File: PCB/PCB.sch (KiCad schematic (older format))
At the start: 44 parts, among them J1 USB_B, J10 Vapor maker, J11 chamber LED, J2 power 12V, J3 DS18B20, J4 NEXTION 2.8\", J5 4pin FAN, J6 4pin FAN, J7 4pin FAN, J8 Peltiers 12V, J9 Peltiers 3.3V, Q1 IRF530N, Q10 IRFD110, Q11 IRFD110, Q12 IRFD110, Q13 IRFD110, Q14 IRFD110, Q15 IRF530N, Q2 IRF530N, Q3 IRF530N, Q4 IRF530N, Q5 IRF530N, Q6 IRF530N, Q7 IRFD110, Q8 IRFD110, Q9 IRFD110, U1 CH340G, U2 ESP32-WROOM-32, U3 LF33CDT, U4 L7805, Y1 12MHz

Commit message: PCB General UPGRADE
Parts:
- removed J11: chamber LED, TerminalBlock_WAGO:TerminalBlock_WAGO_804-102_1x02_P5.00mm_45Degree, symbol Connector_Generic:Conn_01x02
- removed Q10, Q11, Q12, Q13, Q14, Q7, Q8, Q9: IRFD110, Package_DIP:Vishay_HVM-DIP-3_W7.62mm, symbol Transistor_FET:IRF40DM229
- removed Q15: IRF530N, Package_TO_SOT_THT:TO-220-3_Vertical, symbol Transistor_FET:IRF540N
- added H1, H2, H3, H4: MountingHole_Pad, MountingHole:MountingHole_3.2mm_M3_Pad_Via, symbol Mechanical:MountingHole_Pad
- added J11: LED + Pump, TerminalBlock_WAGO:TerminalBlock_WAGO_236-104_1x04_P5.00mm_45Degree, symbol Connector_Generic:Conn_01x04
- added J12: I2C, Connector_PinHeader_2.54mm:PinHeader_1x04_P2.54mm_Horizontal, symbol Connector_Generic:Conn_01x04
- added Q10, Q11, Q12, Q13, Q14, Q15, Q7, Q8, Q9: TSM2302, Package_TO_SOT_SMD:SOT-23, symbol Transistor_FET:ZXMN2A01F
- added Q16, Q17: IRF530N, Package_TO_SOT_THT:TO-220-3_Vertical, symbol Transistor_FET:IRF540N
- added R8: 5k6, Resistor_SMD:R_1206_3216Metric_Pad1.42x1.75mm_HandSolder, symbol Device:R
- J10, J8, J9: footprint Connector_Phoenix_GMSTB:PhoenixContact_GMSTBVA_2,5_4-G-7,62_1x04_P7.62mm_Vertical -> TerminalBlock_WAGO:TerminalBlock_WAGO_236-104_1x04_P5.00mm_45Degree
- R1, R2, R3, R4, R5, R6, R7: footprint Resistor_THT:R_Axial_DIN0207_L6.3mm_D2.5mm_P10.16mm_Horizontal -> Resistor_SMD:R_1206_3216Metric_Pad1.42x1.75mm_HandSolder
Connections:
- wire segments 193 -> 212

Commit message: pcb update
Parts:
- removed C3, C6: 0.1uF, Capacitor_SMD:C_1206_3216Metric, symbol Device:C
- removed C4: 2.2uF, Capacitor_THT:CP_Radial_D5.0mm_P2.00mm, symbol Device:CP
- removed C5: 0.33uF, Capacitor_SMD:C_1206_3216Metric, symbol Device:C
- removed H1, H2, H3, H4: MountingHole_Pad, MountingHole:MountingHole_3.2mm_M3_Pad_Via, symbol Mechanical:MountingHole_Pad
- removed J10: Vapor maker, TerminalBlock_WAGO:TerminalBlock_WAGO_236-104_1x04_P5.00mm_45Degree, symbol Connector_Generic:Conn_01x04
- removed J11: LED + Pump, TerminalBlock_WAGO:TerminalBlock_WAGO_236-104_1x04_P5.00mm_45Degree, symbol Connector_Generic:Conn_01x04
- removed J12: I2C, Connector_PinHeader_2.54mm:PinHeader_1x04_P2.54mm_Horizontal, symbol Connector_Generic:Conn_01x04
- removed J2: power 12V, Connector_PinHeader_2.54mm:PinHeader_1x03_P2.54mm_Horizontal, symbol Connector_Generic:Conn_01x03
- removed J3: DS18B20, Connector_PinHeader_2.54mm:PinHeader_1x03_P2.54mm_Horizontal, symbol Connector_Generic:Conn_01x03
- removed J4: NEXTION 2.8\", Connector_PinHeader_2.54mm:PinHeader_1x04_P2.54mm_Horizontal, symbol Connector_Generic:Conn_01x04
- removed J5, J6, J7: 4pin FAN, Connector:FanPinHeader_1x04_P2.54mm_Vertical, symbol Connector_Generic:Conn_01x04
- removed J8: Peltiers 12V, TerminalBlock_WAGO:TerminalBlock_WAGO_236-104_1x04_P5.00mm_45Degree, symbol Connector_Generic:Conn_01x04
- removed J9: Peltiers 3.3V, TerminalBlock_WAGO:TerminalBlock_WAGO_236-104_1x04_P5.00mm_45Degree, symbol Connector_Generic:Conn_01x04
- removed Q1, Q16, Q17, Q2, Q3, Q4, Q5, Q6: IRF530N, Package_TO_SOT_THT:TO-220-3_Vertical, symbol Transistor_FET:IRF540N
- removed Q10, Q11, Q12, Q13, Q14, Q15, Q7, Q8, Q9: TSM2302, Package_TO_SOT_SMD:SOT-23, symbol Transistor_FET:ZXMN2A01F
- removed R1, R2, R3, R4, R5, R6, R7, R8: 5k6, Resistor_SMD:R_1206_3216Metric_Pad1.42x1.75mm_HandSolder, symbol Device:R
- removed U1: CH340G, Package_SO:SOP-16_4.4x10.4mm_P1.27mm, symbol Interface_USB:CH340G
- removed U2: ESP32-WROOM-32, RF_Module:ESP32-WROOM-32, symbol RF_Module:ESP32-WROOM-32
- removed U3: LF33CDT, Package_TO_SOT_SMD:TO-252-2, symbol Regulator_Linear:LF33_TO220
- removed U4: L7805, Package_TO_SOT_SMD:TO-252-2, symbol Regulator_Linear:L7805
- removed Y1: 12MHz, Crystal:Crystal_HC49-U_Vertical, symbol Device:Crystal
- added CH340G1: CH340G, Package_SO:SOIC-16_3.9x9.9mm_P1.27mm, symbol Interface_USB:CH340G
- added U1: ESP32-WROOM-32, RF_Module:ESP32-WROOM-32, symbol RF_Module:ESP32-WROOM-32
- added X1: 12MHz, Crystals:Crystal_SMD_HC49-SD_HandSoldering, symbol Device:Crystal
- added power_12V1: Conn_01x03, Mlab_Pin_Headers:Straight_2x03, symbol Connector_Generic:Conn_01x03
- C1, C2: value 22pF -> 22p; footprint Capacitor_SMD:C_1206_3216Metric -> Capacitors_SMD:C_1206_HandSoldering
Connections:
- net labels added: +12V, +3.3V, +5V, DTR, RTS, RXD, TXD, usb_N, usb_P
- wire segments 212 -> 37

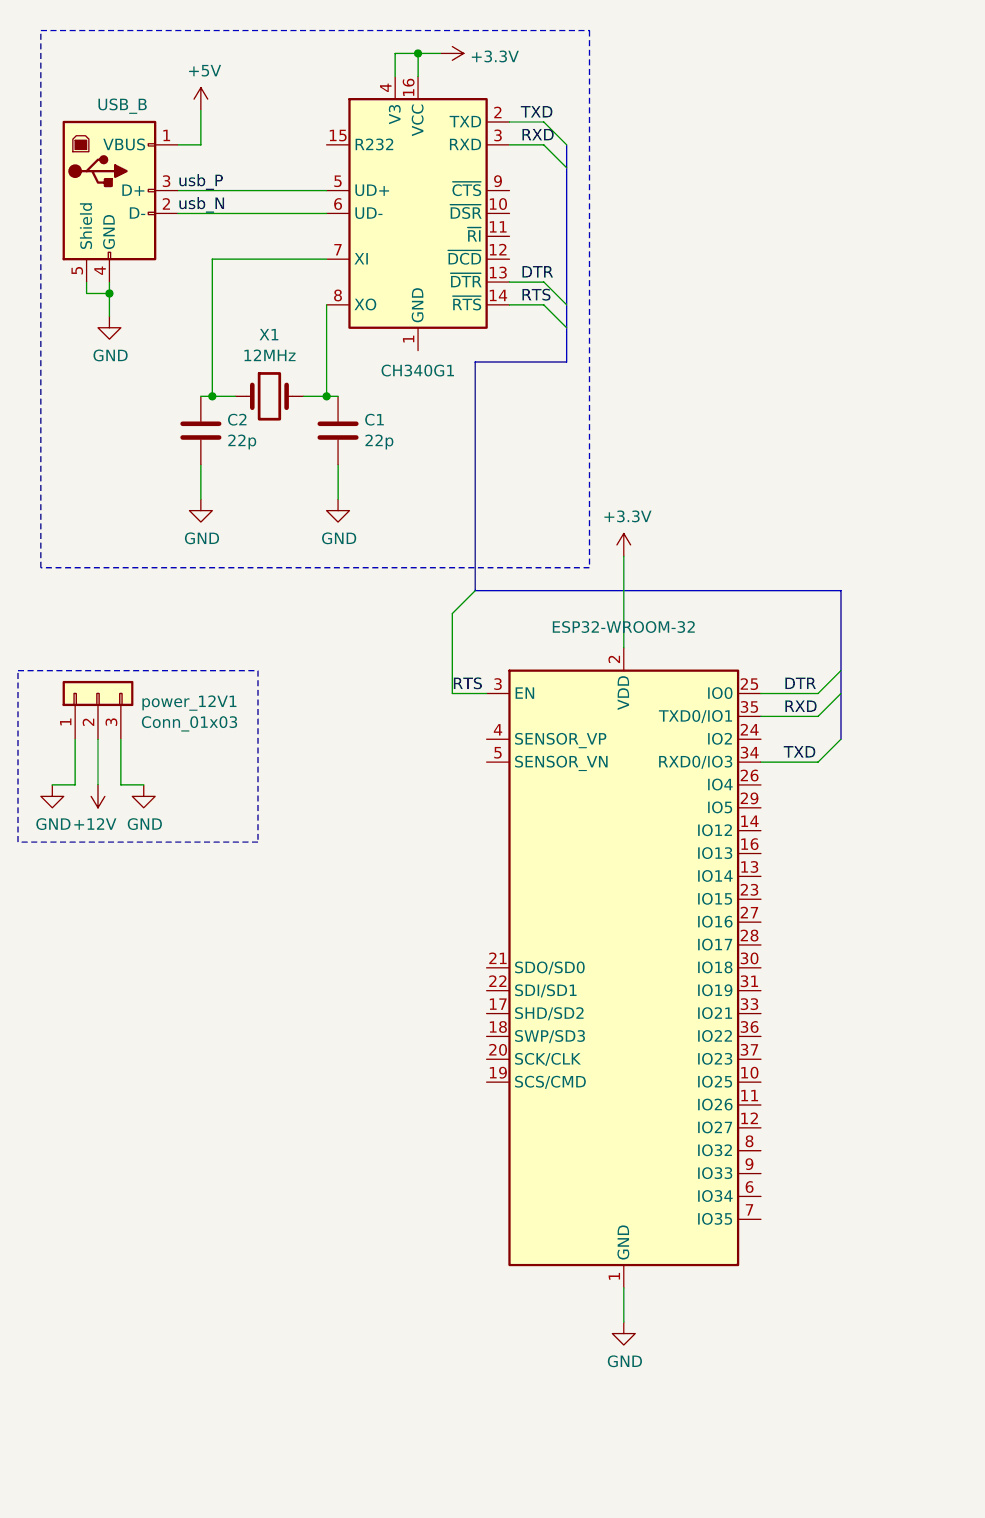
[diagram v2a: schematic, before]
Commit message: pcb
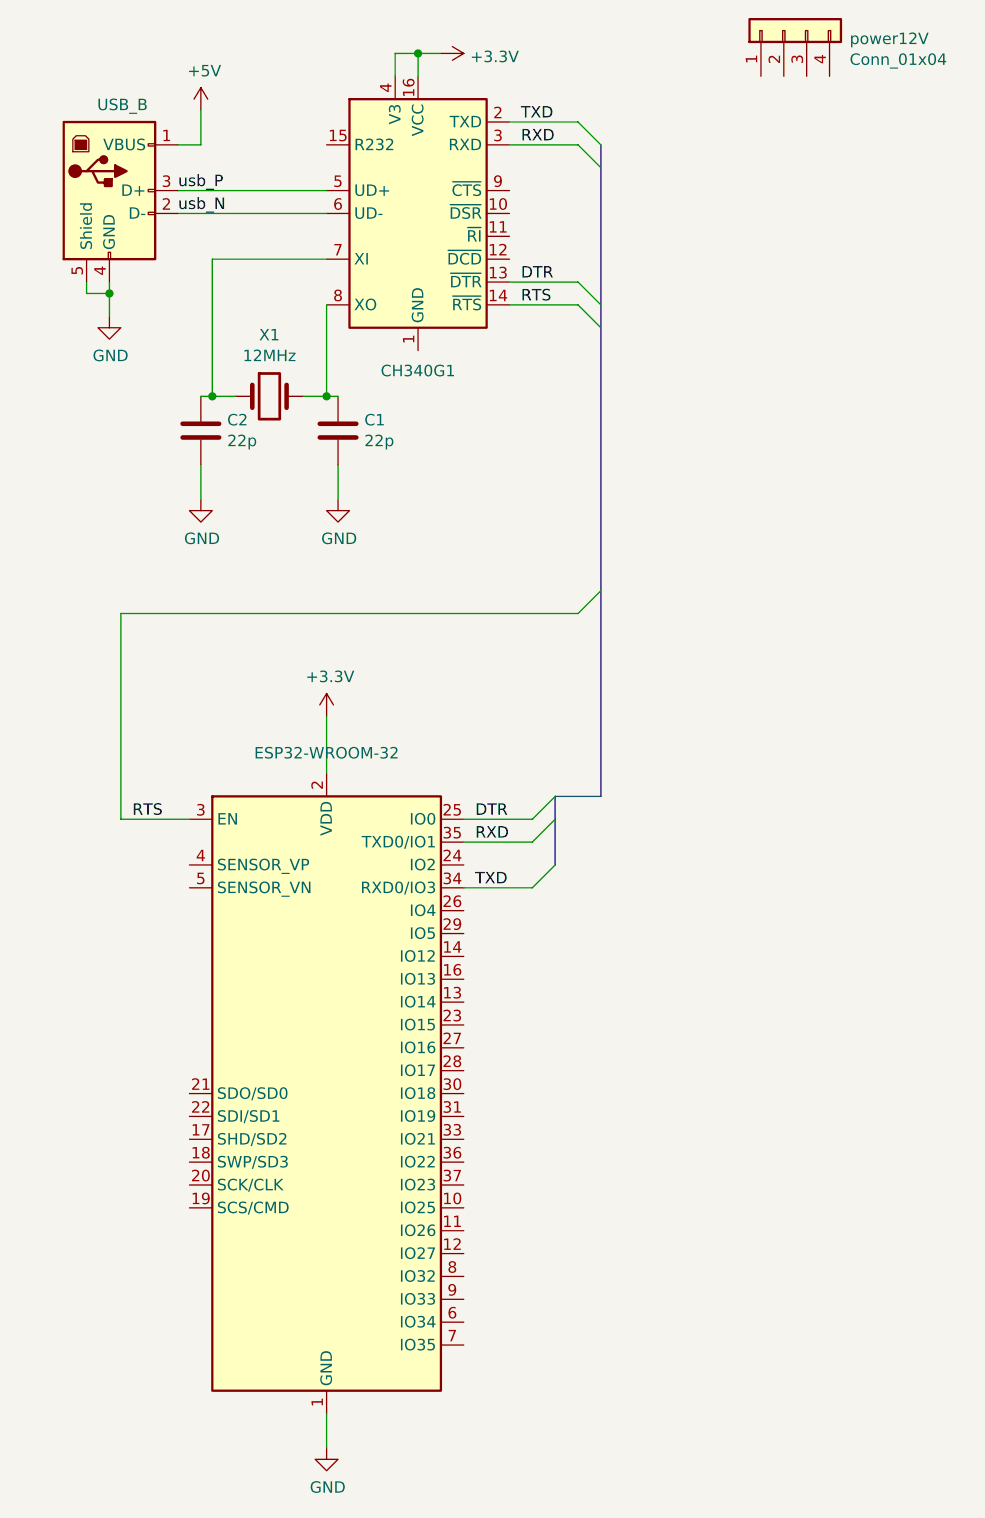
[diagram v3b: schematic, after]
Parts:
- removed power_12V1: Conn_01x03, Mlab_Pin_Headers:Straight_2x03, symbol Connector_Generic:Conn_01x03
- added power12V: Conn_01x04, Mlab_Pin_Headers:Straight_2x04, symbol Connector_Generic:Conn_01x04
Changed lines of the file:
@@
 EESchema Schematic File Version 4
-LIBS:PCB-cache
 EELAYER 30 0
 EELAYER END
@@
 usb_N
 $Comp
-L RF_Module:ESP32-WROOM-32 U1
-U 1 1 5DA32DFA
-P 3700 5150
-F 0 "U1" H 3700 6731 50  0001 C CNN
-F 1 "ESP32-WROOM-32" H 3700 6639 50  0000 C CNN
-F 2 "RF_Module:ESP32-WROOM-32" H 3700 3650 50  0001 C CNN
-F 3 "https://www.espressif.com/sites/default/files/documentation/esp32-wroom-32_datasheet_en.pdf" H 3400 5200 50  0001 C CNN
-	1    3700 5150
-	1    0    0    -1
-$EndComp
-$Comp
 L Device:Crystal X1
 U 1 1 5DA400F9
@@
 Wire Wire Line
 	1450 2200 1450 2150
-Entry Wire Line
-	3350 1450 3450 1550
-Entry Wire Line
-	3350 1550 3450 1650
-Entry Wire Line
-	3350 2150 3450 2250
-Entry Wire Line
-	3350 2250 3450 2350
-Wire Wire Line
-	3200 1450 3350 1450
-Wire Wire Line
-	3200 1550 3350 1550
-Wire Wire Line
-	3200 2150 3350 2150
-Wire Wire Line
-	3200 2250 3350 2250
-Text Label 3250 1450 0    50   ~ 0
-TXD
-Text Label 3250 1550 0    50   ~ 0
-RXD
-Text Label 3250 2150 0    50   ~ 0
-DTR
-Text Label 3250 2250 0    50   ~ 0
-RTS
-Wire Wire Line
-	3100 3950 2950 3950
-Wire Wire Line
-	2950 3950 2950 3600
-Entry Wire Line
-	2950 3600 3050 3500
-Wire Wire Line
-	4300 4050 4550 4050
-Wire Wire Line
-	4300 4250 4550 4250
-Entry Wire Line
-	4550 4050 4650 3950
-Entry Wire Line
-	4550 4250 4650 4150
-Wire Bus Line
-	4650 3500 3050 3500
-Wire Bus Line
-	3050 3500 3050 2500
-Wire Bus Line
-	3050 2500 3450 2500
-Text Label 4400 4250 0    50   ~ 0
-TXD
-Text Label 4400 4050 0    50   ~ 0
-RXD
-Text Label 2950 3950 0    50   ~ 0
-RTS
-Wire Wire Line
-	4300 3950 4550 3950
-Entry Wire Line
-	4550 3950 4650 3850
-Text Label 4400 3950 0    50   ~ 0
-DTR
-$Comp
-L power:+3.3V #PWR0108
-U 1 1 5DA62BDB
-P 3700 3350
-F 0 "#PWR0108" H 3700 3200 50  0001 C CNN
-F 1 "+3.3V" H 3715 3523 50  0000 C CNN
-F 2 "" H 3700 3350 50  0001 C CNN
-F 3 "" H 3700 3350 50  0001 C CNN
-	1    3700 3350
-	1    0    0    -1
-$EndComp
-Wire Wire Line
-	3700 3750 3700 3350
-$Comp
-L power:GND #PWR0109
-U 1 1 5DA64609
-P 3700 6700
-F 0 "#PWR0109" H 3700 6450 50  0001 C CNN
-F 1 "GND" H 3705 6527 50  0000 C CNN
-F 2 "" H 3700 6700 50  0001 C CNN
-F 3 "" H 3700 6700 50  0001 C CNN
-	1    3700 6700
-	1    0    0    -1
-$EndComp
-Wire Wire Line
-	3700 6700 3700 6550
-$Comp
-L Connector_Generic:Conn_01x03 power_12V1
-U 1 1 5DA737E0
-P 1400 3950
-F 0 "power_12V1" V 1364 3762 50  0000 R CNN
-F 1 "Conn_01x03" V 1273 3762 50  0000 R CNN
-F 2 "Mlab_Pin_Headers:Straight_2x03" H 1400 3950 50  0001 C CNN
-F 3 "~" H 1400 3950 50  0001 C CNN
-	1    1400 3950
-	0    -1   -1   0
-$EndComp
-$Comp
-L power:+12V #PWR0101
-U 1 1 5DA7649D
-P 1400 4350
-F 0 "#PWR0101" H 1400 4200 50  0001 C CNN
-F 1 "+12V" H 1415 4523 50  0000 C CNN
-F 2 "" H 1400 4350 50  0001 C CNN
-F 3 "" H 1400 4350 50  0001 C CNN
-	1    1400 4350
-	-1   0    0    1
-$EndComp
-$Comp
-L power:GND #PWR0102
-U 1 1 5DA7684F
-P 1600 4350
-F 0 "#PWR0102" H 1600 4100 50  0001 C CNN
-F 1 "GND" H 1605 4177 50  0000 C CNN
-F 2 "" H 1600 4350 50  0001 C CNN
-F 3 "" H 1600 4350 50  0001 C CNN
-	1    1600 4350
-	1    0    0    -1
-$EndComp
-$Comp
-L power:GND #PWR0103
-U 1 1 5DA76A88
-P 1200 4350
-F 0 "#PWR0103" H 1200 4100 50  0001 C CNN
-F 1 "GND" H 1205 4177 50  0000 C CNN
-F 2 "" H 1200 4350 50  0001 C CNN
-F 3 "" H 1200 4350 50  0001 C CNN
-	1    1200 4350
-	1    0    0    -1
-$EndComp
-Wire Wire Line
-	1400 4350 1400 4150
-Wire Wire Line
-	1300 4150 1300 4350
-Wire Wire Line
-	1300 4350 1200 4350
-Wire Wire Line
-	1500 4150 1500 4350
-Wire Wire Line
-	1500 4350 1600 4350
-Wire Notes Line
-	1050 4600 1050 3850
-Wire Notes Line
-	1050 3850 2100 3850
-Wire Notes Line
-	2100 3850 2100 4600
-Wire Notes Line
-	2100 4600 1050 4600
-Wire Notes Line
-	1150 1050 3550 1050
-Wire Notes Line
-	3550 1050 3550 3400
-Wire Notes Line
-	3550 3400 1150 3400
-Wire Notes Line
-	1150 3400 1150 1050
 $Comp
 L power:+3.3V #PWR?
@@
 Wire Wire Line
 	2800 1250 2800 1150
+Connection ~ 2800 1150
+Wire Wire Line
+	2800 1150 2700 1150
+$Comp
+L Connector_Generic:Conn_01x04 power12V
+U 1 1 5DEF05BC
+P 4400 1050
+F 0 "power12V" V 4364 762 50  0000 R CNN
+F 1 "Conn_01x04" V 4273 762 50  0000 R CNN
+F 2 "Mlab_Pin_Headers:Straight_2x04" H 4400 1050 50  0001 C CNN
+F 3 "~" H 4400 1050 50  0001 C CNN
+	1    4400 1050
+	0    -1   -1   0
+$EndComp
+$Comp
+L RF_Module:ESP32-WROOM-32 U1
+U 1 1 5DA32DFA
+P 2400 5700
+F 0 "U1" H 2400 7281 50  0001 C CNN
+F 1 "ESP32-WROOM-32" H 2400 7189 50  0000 C CNN
+F 2 "RF_Module:ESP32-WROOM-32" H 2400 4200 50  0001 C CNN
+F 3 "https://www.espressif.com/sites/default/files/documentation/esp32-wroom-32_datasheet_en.pdf" H 2100 5750 50  0001 C CNN
+	1    2400 5700
+	1    0    0    -1
+$EndComp
+$Comp
+L power:GND #PWR0109
+U 1 1 5DA64609
+P 2400 7250
+F 0 "#PWR0109" H 2400 7000 50  0001 C CNN
+F 1 "GND" H 2405 7077 50  0000 C CNN
+F 2 "" H 2400 7250 50  0001 C CNN
+F 3 "" H 2400 7250 50  0001 C CNN
+	1    2400 7250
+	1    0    0    -1
+$EndComp
+Wire Wire Line
+	2400 7250 2400 7100
+Wire Wire Line
+	3000 4500 3300 4500
+Wire Wire Line
+	3000 4600 3300 4600
+Wire Wire Line
+	3000 4800 3300 4800
+Wire Wire Line
+	1800 4500 1500 4500
+Wire Wire Line
+	3200 1450 3500 1450
+Wire Wire Line
+	3200 1550 3500 1550
+Wire Wire Line
+	3200 2150 3500 2150
+Wire Wire Line
+	3200 2250 3500 2250
+Text Label 3250 1450 0    50   ~ 0
+TXD
+Text Label 3250 1550 0    50   ~ 0
+RXD
+Text Label 3250 2150 0    50   ~ 0
+DTR
+Text Label 3250 2250 0    50   ~ 0
+RTS
+Text Label 1550 4500 0    50   ~ 0
+RTS
+Text Label 3050 4500 0    50   ~ 0
+DTR
+Text Label 3050 4600 0    50   ~ 0
+RXD
+Text Label 3050 4800 0    50   ~ 0
+TXD
+Entry Wire Line
+	3300 4800 3400 4700
+Entry Wire Line
+	3300 4600 3400 4500
+Entry Wire Line
+	3300 4500 3400 4400
+Entry Wire Line
+	3500 2250 3600 2350
+Entry Wire Line
+	3500 2150 3600 2250
+Entry Wire Line
+	3500 1550 3600 1650
+Entry Wire Line
+	3500 1450 3600 1550
 Wire Bus Line
-	4650 3500 4650 4150
+	3600 4400 3400 4400
+Wire Wire Line
+	1500 4500 1500 3600
+Entry Wire Line
+	3500 3600 3600 3500
+Wire Wire Line
+	1500 3600 3500 3600
+$Comp
+L power:+3.3V #PWR?
+U 1 1 5DF14F2C
+P 2400 4050
+F 0 "#PWR?" H 2400 3900 50  0001 C CNN
+F 1 "+3.3V" H 2415 4223 50  0000 C CNN
+F 2 "" H 2400 4050 50  0001 C CNN
+F 3 "" H 2400 4050 50  0001 C CNN
+	1    2400 4050
+	1    0    0    -1
+$EndComp
+Wire Wire Line
+	2400 4300 2400 4050
 Wire Bus Line
-	3450 1550 3450 2500
-Connection ~ 2800 1150
-Wire Wire Line
-	2800 1150 2700 1150
+	3400 4400 3400 4700
+Wire Bus Line
+	3600 1550 3600 4400
 $EndSCHEMATC

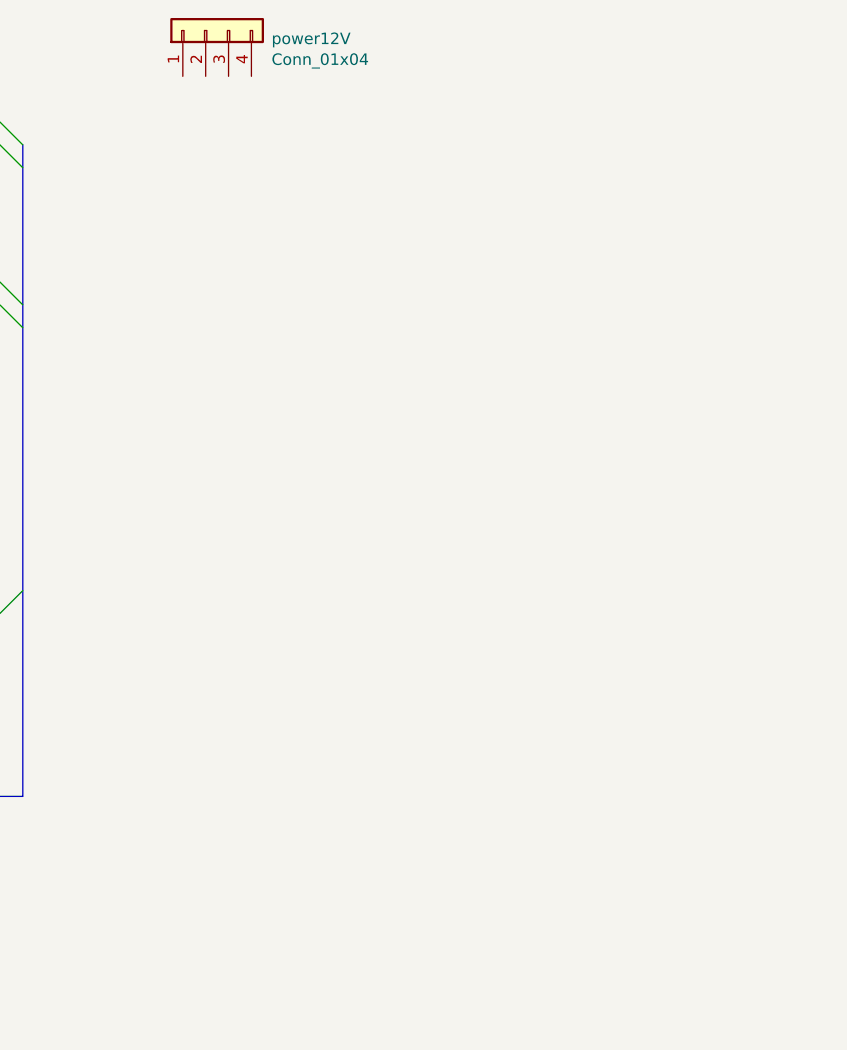
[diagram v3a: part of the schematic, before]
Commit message: pcb, power and 3v3
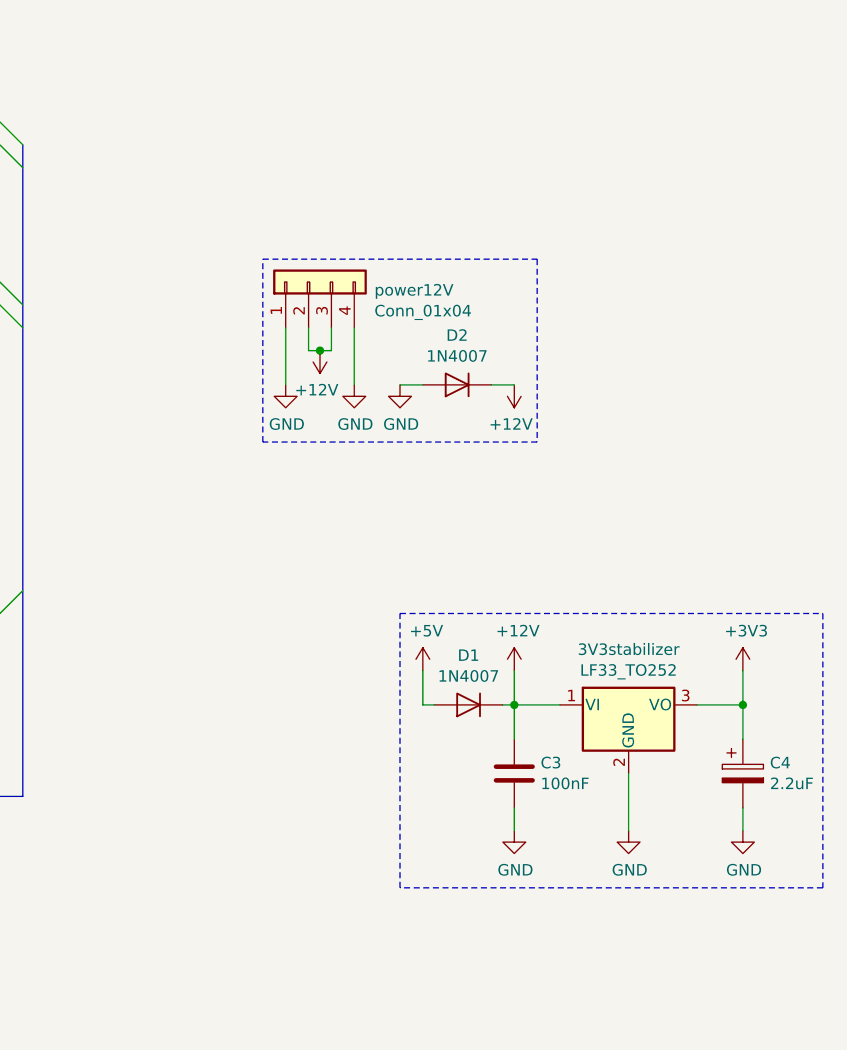
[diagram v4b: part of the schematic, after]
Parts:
- added 3V3stabilizer: LF33_TO252, Package_TO_SOT_SMD:TO-252-2, symbol Regulator_Linear:LF33_TO252
- added C3: 100nF, Capacitor_SMD:C_1206_3216Metric_Pad1.42x1.75mm_HandSolder, symbol Device:C
- added C4: 2.2uF, Capacitor_SMD:CP_Elec_4x5.4, symbol Device:CP
- added D1: 1N4007, Diode_SMD:D_SMA_Handsoldering, symbol Diode:1N4007
- added D2: 1N4007, Diodes_SMD:D_SMA_Handsoldering, symbol Diode:1N4007
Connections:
- net +3V3: now also 3V3stabilizer.3 (VO), C4.1
- net +5V: now also D1.2 (A)
- net GND: now also power12V.1 (Pin_1), power12V.4 (Pin_4), 3V3stabilizer.2 (GND), C3.2, C4.2, D2.2 (A)
- net +12V: now reaches power12V.2 (Pin_2)
- net +12V: now also power12V.3 (Pin_3), 3V3stabilizer.1 (VI), C3.1, D1.1 (K), D2.1 (K)
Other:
- moved on the sheet: power12V
